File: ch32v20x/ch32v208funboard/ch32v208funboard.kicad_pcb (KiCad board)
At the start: 2 copper layers, 40.6 x 38.1 mm, 21 parts, among them J1 HDR, J2 PGM, J3 USB_C_Receptacle_USB2.0, J4 HDR, U1 CH32V208GBU6, U3 XC6206P332, Y2 32MHz

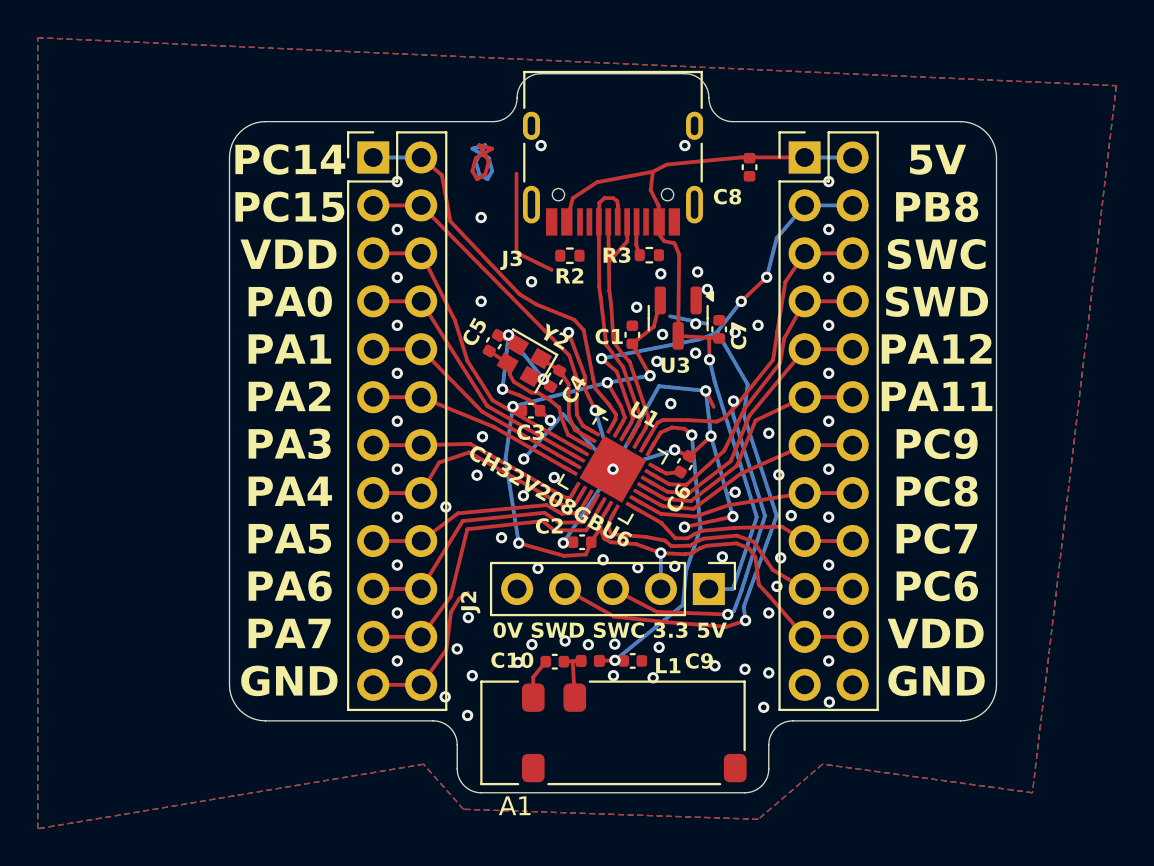
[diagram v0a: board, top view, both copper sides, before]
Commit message: Bump 208 board
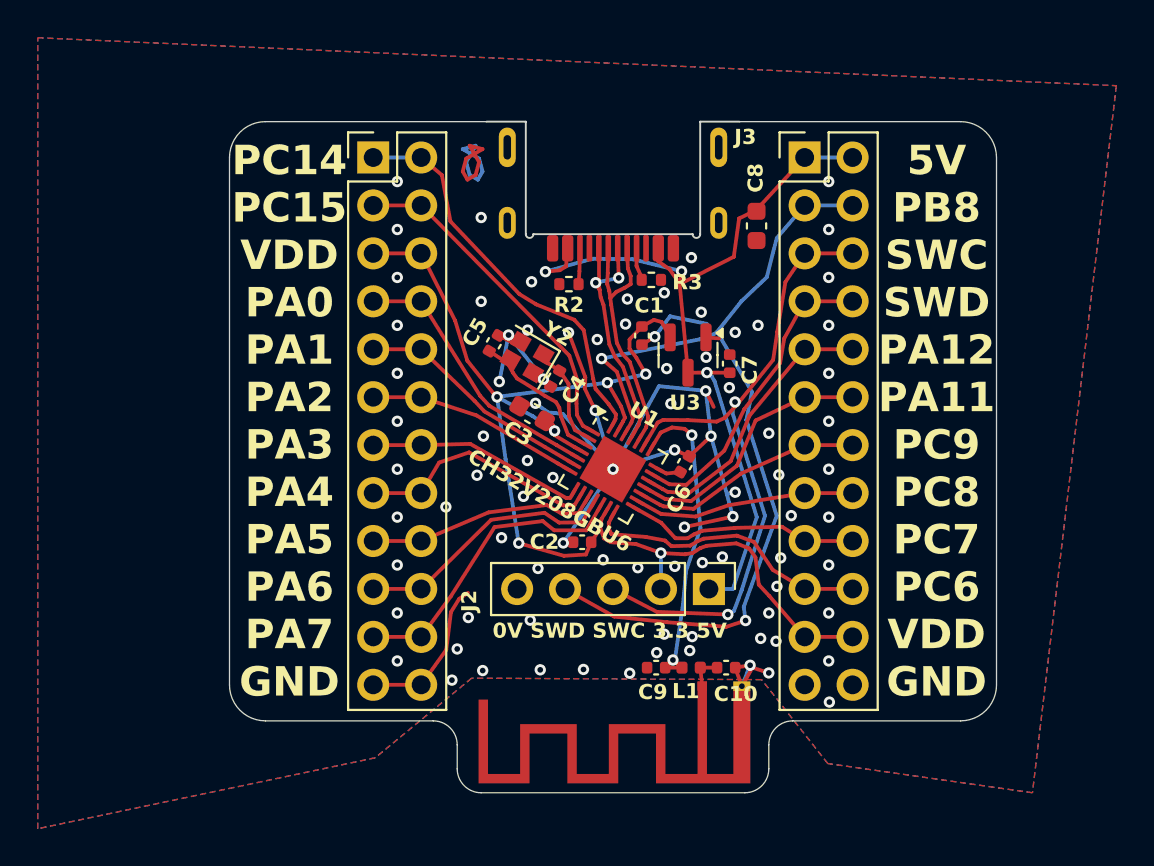
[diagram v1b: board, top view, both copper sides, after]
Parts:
- A1: footprint RF_Antenna:Abracon_PRO-OB-440 -> RF_Antenna:Texas_SWRA117D_2.4GHz_Right
- C3, C8: value 1u -> 10u; footprint Capacitor_SMD:C_0402_1005Metric -> Capacitor_SMD:C_0603_1608Metric
- J3: footprint cnhardware:USB_C_MOD_Receptacle_HRO_TYPE-C-31-M-12 -> cnhardware:USB_C_TIGHT_IN_BOARD_161N-4BC21665
- moved C10 9.08 mm to (126.0, 85.4), turned to 0 degrees
- moved L1 5.36 mm to (124.2, 85.4), turned to 0 degrees
- moved A1 5.34 mm to (124.7, 86.4), turned to 180 degrees
- moved C8 3.13 mm to (127.6, 62.0)
- moved U3 2.02 mm to (124.0, 68.9)
- moved C7 1.90 mm to (126.2, 69.3)
- moved R2 1.51 mm to (117.7, 65.1)
- moved R3 1.31 mm to (122.0, 64.9)
- moved C9 1.29 mm to (122.3, 85.4), turned to 180 degrees
- moved C1 0.51 mm to (121.5, 67.8), turned to -90 degrees
- moved Y2 0.25 mm to (115.5, 69.0)
- moved C3 0.16 mm to (115.7, 72.0), turned to 150 degrees
- moved J3 0.09 mm to (120.0, 57.9)
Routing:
- net GND: track 74.9 -> 69.8 mm, vias 88 -> 89
- net +5V: track 43.2 -> 45.5 mm, vias 1 -> 3
- net CC2: track 0.00 -> 1.90 mm
- net VDD: track 64.7 -> 66.3 mm, vias 5 -> 6
- net D+: track 15.2 -> 13.8 mm, vias 0 -> 2
- net Net-(A1-Pad1): track 2.84 -> 1.88 mm
- net Net-(U1-ANT): track 17.9 -> 17.1 mm
- net Net-(J1-Pin_21): track 16.9 -> 16.2 mm
- net D-: track 14.7 -> 14.0 mm
- net Net-(J1-Pin_19): track 14.6 -> 14.1 mm
- net PA13/SWD: vias 4 -> 2
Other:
- board size 40.6 x 38.1 mm -> 40.6 x 35.6 mm
